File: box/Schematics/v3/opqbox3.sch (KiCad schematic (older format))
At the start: 2 parts, among them J1 Conn_01x02_Male, J2 Conn_01x02_Male

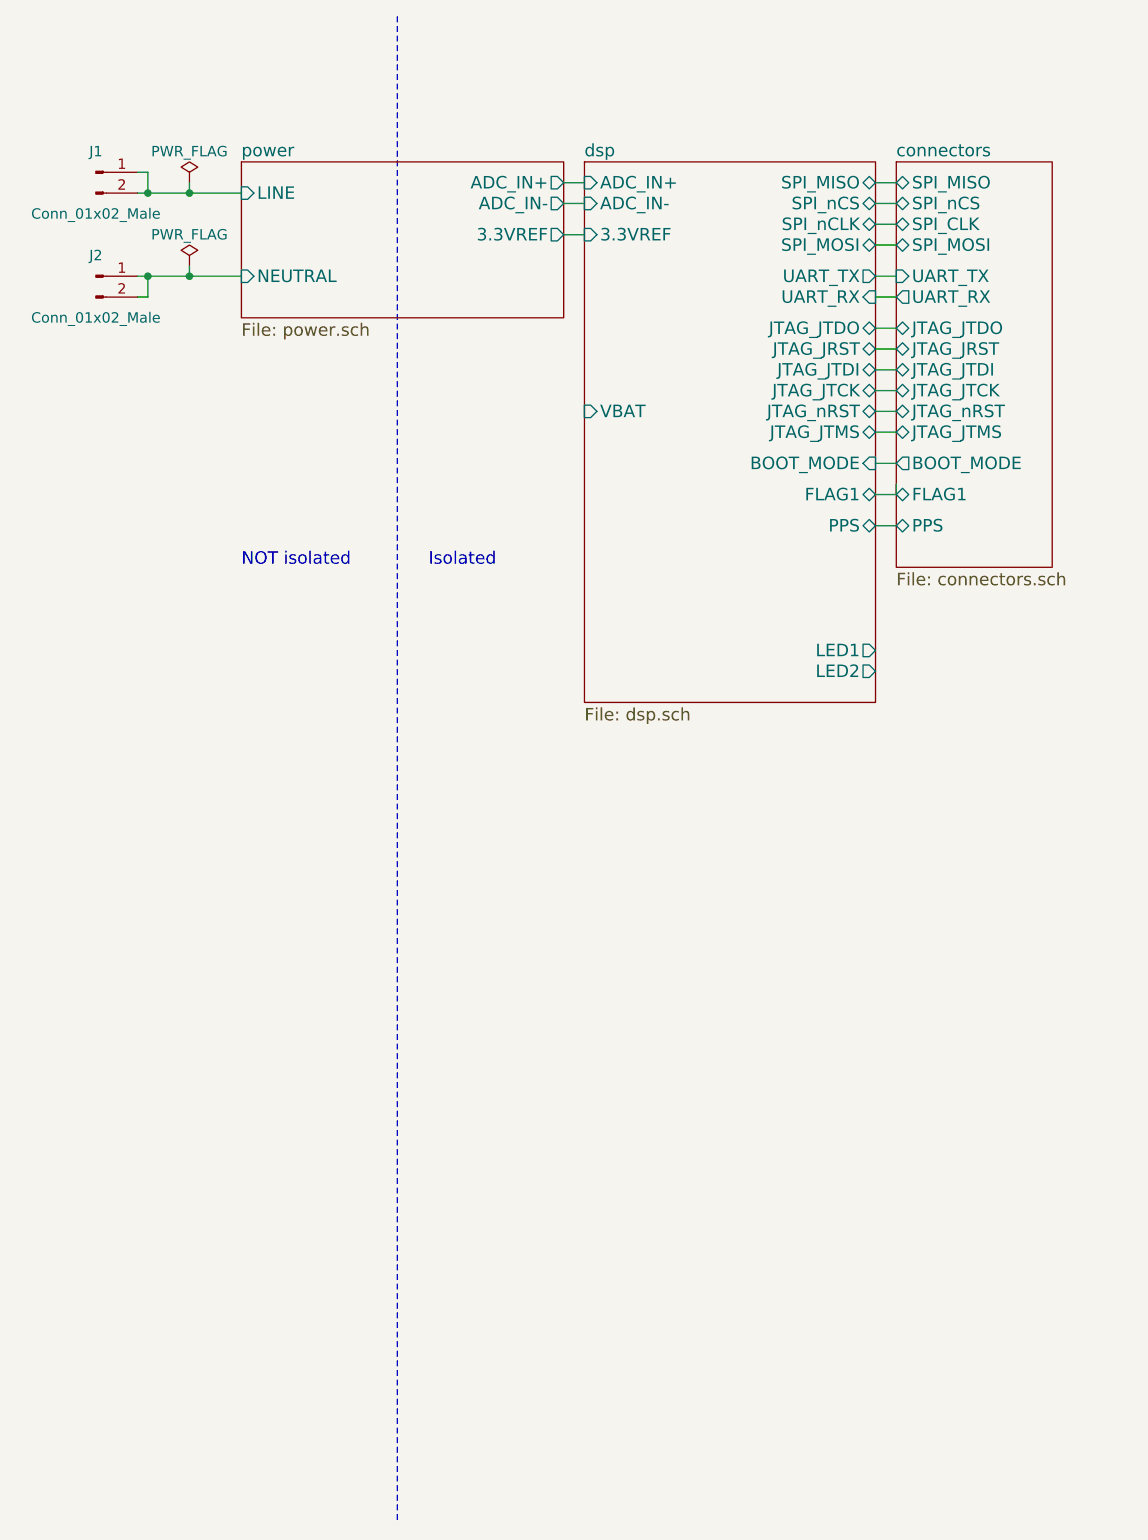
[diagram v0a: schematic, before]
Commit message: create io schematics
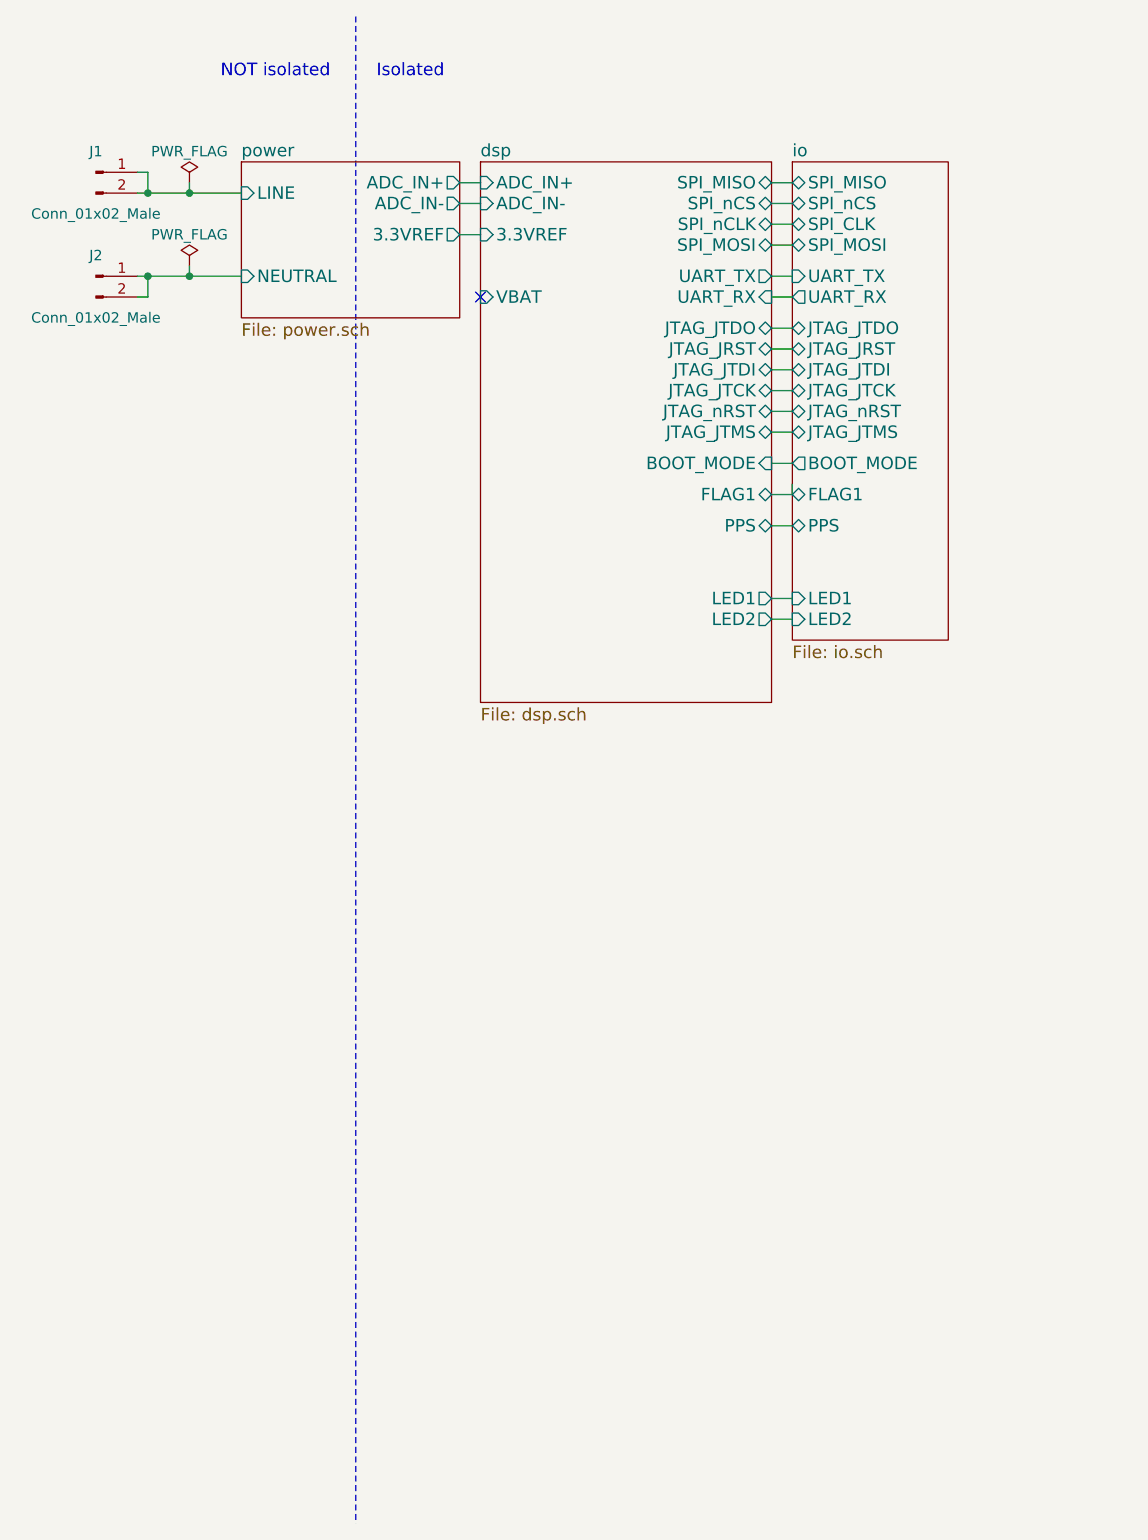
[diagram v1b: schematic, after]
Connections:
- no-connect marks 0 -> 1
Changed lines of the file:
@@
 $EndDescr
 $Sheet
-S 2150 1200 1550 750
+S 2150 1200 1050 750
 U 5A829EE9
 F0 "power" 60
@@
 F2 "LINE" I L 2150 1350 60
 F3 "NEUTRAL" I L 2150 1750 60
-F4 "3.3VREF" O R 3700 1550 60
-F5 "ADC_IN-" O R 3700 1400 60
-F6 "ADC_IN+" O R 3700 1300 60
+F4 "3.3VREF" O R 3200 1550 60
+F5 "ADC_IN-" O R 3200 1400 60
+F6 "ADC_IN+" O R 3200 1300 60
 $EndSheet
 $Comp
@@
 	1    0    0    -1
 $EndComp
-Text Notes 3050 3150 0    60   ~ 0
+Text Notes 2800 800  0    60   ~ 0
 Isolated
-Text Notes 2150 3150 0    60   ~ 0
+Text Notes 2050 800  0    60   ~ 0
 NOT isolated
+$Sheet
+S 4800 1200 750  2300
+U 5A8506F3
+F0 "io" 60
+F1 "io.sch" 60
+F2 "SPI_MISO" B L 4800 1300 60
+F3 "SPI_MOSI" B L 4800 1600 60
+F4 "SPI_nCS" B L 4800 1400 60
+F5 "SPI_CLK" B L 4800 1500 60
+F6 "JTAG_nRST" B L 4800 2400 60
+F7 "BOOT_MODE" O L 4800 2650 60
+F8 "UART_RX" O L 4800 1850 60
+F9 "UART_TX" I L 4800 1750 60
+F10 "FLAG1" B L 4800 2800 60
+F11 "JTAG_JRST" B L 4800 2100 60
+F12 "JTAG_JTCK" B L 4800 2300 60
+F13 "JTAG_JTDI" B L 4800 2200 60
+F14 "JTAG_JTDO" B L 4800 2000 60
+F15 "JTAG_JTMS" B L 4800 2500 60
+F16 "PPS" B L 4800 2950 60
+F17 "LED1" I L 4800 3300 60
+F18 "LED2" I L 4800 3400 60
+$EndSheet
+$Sheet
+S 3300 1200 1400 2600
+U 5A835DDE
+F0 "dsp" 60
+F1 "dsp.sch" 60
+F2 "BOOT_MODE" I R 4700 2650 60
+F3 "VBAT" I L 3300 1850 60
+F4 "SPI_MISO" B R 4700 1300 60
+F5 "LED1" O R 4700 3300 60
+F6 "FLAG1" B R 4700 2800 60
+F7 "ADC_IN+" I L 3300 1300 60
+F8 "SPI_nCS" B R 4700 1400 60
+F9 "SPI_nCLK" B R 4700 1500 60
+F10 "SPI_MOSI" B R 4700 1600 60
+F11 "ADC_IN-" I L 3300 1400 60
+F12 "LED2" O R 4700 3400 60
+F13 "JTAG_JTDO" B R 4700 2000 60
+F14 "JTAG_JRST" B R 4700 2100 60
+F15 "JTAG_JTDI" B R 4700 2200 60
+F16 "JTAG_JTCK" B R 4700 2300 60
+F17 "JTAG_nRST" B R 4700 2400 60
+F18 "JTAG_JTMS" B R 4700 2500 60
+F19 "3.3VREF" I L 3300 1550 60
+F20 "UART_RX" I R 4700 1850 60
+F21 "UART_TX" O R 4700 1750 60
+F22 "PPS" B R 4700 2950 60
+$EndSheet
 Wire Notes Line
-	2900 500  2900 7750
+	2700 500  2700 7750
 Wire Wire Line
 	1650 1250 1700 1250
@@
 	1900 1300 1900 1350
 Connection ~ 1900 1350
-$Sheet
-S 5300 1200 750  1950
-U 5A8506F3
-F0 "connectors" 60
-F1 "connectors.sch" 60
-F2 "SPI_MISO" B L 5300 1300 60
-F3 "SPI_MOSI" B L 5300 1600 60
-F4 "SPI_nCS" B L 5300 1400 60
-F5 "SPI_CLK" B L 5300 1500 60
-F6 "JTAG_nRST" B L 5300 2400 60
-F7 "BOOT_MODE" O L 5300 2650 60
-F8 "UART_RX" O L 5300 1850 60
-F9 "UART_TX" I L 5300 1750 60
-F10 "FLAG1" B L 5300 2800 60
-F11 "JTAG_JRST" B L 5300 2100 60
-F12 "JTAG_JTCK" B L 5300 2300 60
-F13 "JTAG_JTDI" B L 5300 2200 60
-F14 "JTAG_JTDO" B L 5300 2000 60
-F15 "JTAG_JTMS" B L 5300 2500 60
-F16 "PPS" B L 5300 2950 60
-$EndSheet
 Wire Wire Line
-	5300 2750 5300 2800
+	4800 2750 4800 2800
 Wire Wire Line
-	5300 2800 5200 2800
+	4800 2800 4700 2800
 Wire Wire Line
-	5200 2650 5300 2650
+	4700 2650 4800 2650
 Wire Wire Line
-	5200 2500 5300 2500
+	4700 2500 4800 2500
 Wire Wire Line
-	5200 2400 5300 2400
+	4700 2400 4800 2400
 Wire Wire Line
-	5200 2300 5300 2300
+	4700 2300 4800 2300
 Wire Wire Line
-	5200 2200 5300 2200
+	4700 2200 4800 2200
 Wire Wire Line
-	5200 2100 5300 2100
+	4700 2100 4800 2100
 Wire Wire Line
-	5200 2000 5300 2000
+	4700 2000 4800 2000
 Wire Wire Line
-	5200 1850 5300 1850
+	4700 1850 4800 1850
 Wire Wire Line
-	5300 1750 5200 1750
+	4800 1750 4700 1750
 Wire Wire Line
-	5200 1600 5300 1600
+	4700 1600 4800 1600
 Wire Wire Line
-	5200 1500 5300 1500
+	4700 1500 4800 1500
 Wire Wire Line
-	5200 1400 5300 1400
+	4700 1400 4800 1400
 Wire Wire Line
-	5200 1300 5300 1300
-$Sheet
-S 3800 1200 1400 2600
-U 5A835DDE
-F0 "dsp" 60
-F1 "dsp.sch" 60
-F2 "BOOT_MODE" I R 5200 2650 60
-F3 "VBAT" I L 3800 2400 60
-F4 "SPI_MISO" B R 5200 1300 60
-F5 "LED1" O R 5200 3550 60
-F6 "FLAG1" B R 5200 2800 60
-F7 "ADC_IN+" I L 3800 1300 60
-F8 "SPI_nCS" B R 5200 1400 60
-F9 "SPI_nCLK" B R 5200 1500 60
-F10 "SPI_MOSI" B R 5200 1600 60
-F11 "ADC_IN-" I L 3800 1400 60
-F12 "LED2" O R 5200 3650 60
-F13 "JTAG_JTDO" B R 5200 2000 60
-F14 "JTAG_JRST" B R 5200 2100 60
-F15 "JTAG_JTDI" B R 5200 2200 60
-F16 "JTAG_JTCK" B R 5200 2300 60
-F17 "JTAG_nRST" B R 5200 2400 60
-F18 "JTAG_JTMS" B R 5200 2500 60
-F19 "3.3VREF" I L 3800 1550 60
-F20 "UART_RX" I R 5200 1850 60
-F21 "UART_TX" O R 5200 1750 60
-F22 "PPS" B R 5200 2950 60
-$EndSheet
+	4700 1300 4800 1300
 Wire Wire Line
-	5200 2950 5300 2950
+	4700 2950 4800 2950
 Wire Wire Line
-	3700 1300 3800 1300
+	3200 1300 3300 1300
 Wire Wire Line
-	3700 1400 3800 1400
+	3200 1400 3300 1400
 Wire Wire Line
-	3700 1550 3800 1550
+	3200 1550 3300 1550
+Wire Wire Line
+	4700 3300 4800 3300
+Wire Wire Line
+	4700 3400 4800 3400
+NoConn ~ 3300 1850
 $EndSCHEMATC
